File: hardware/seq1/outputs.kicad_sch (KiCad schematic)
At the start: 18 parts, among them J1 AudioJack2_SwitchT, J2 AudioJack2_SwitchT, J4 AudioJack2_SwitchT, U6 TL074

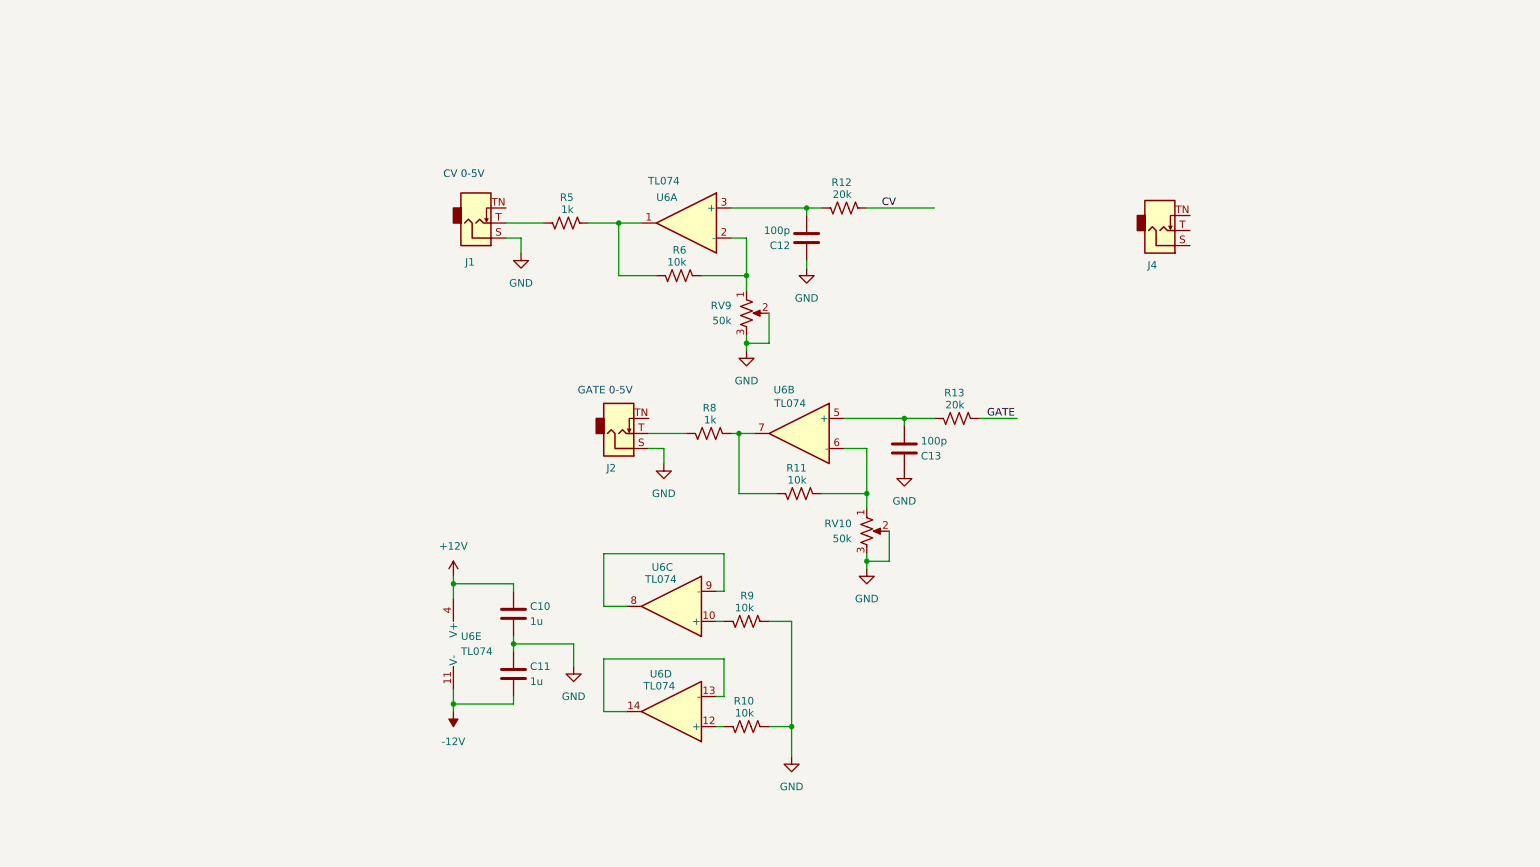
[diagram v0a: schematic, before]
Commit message: schematic and layout for v1 board
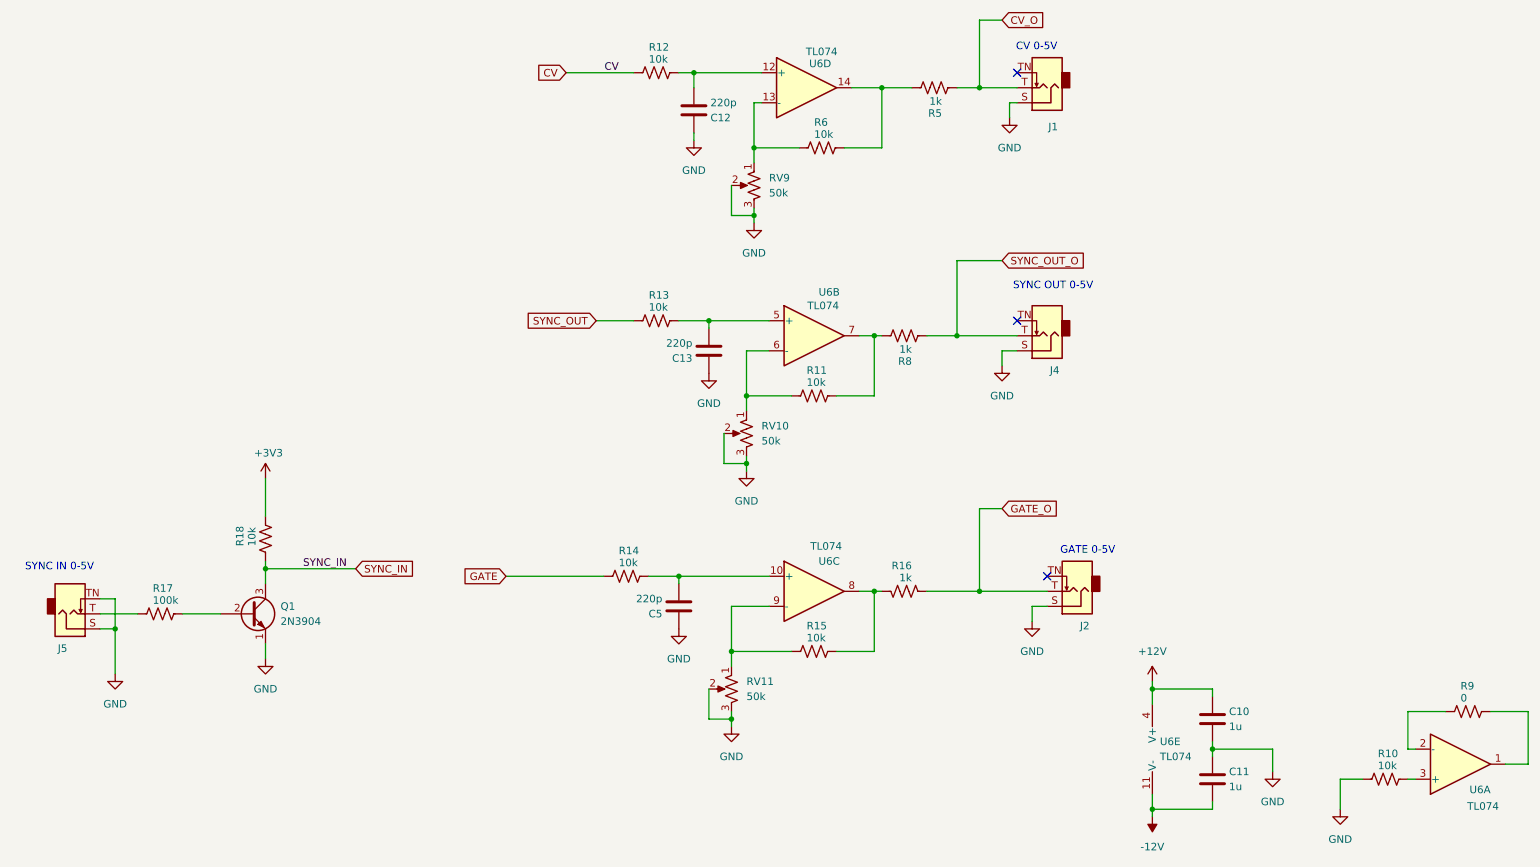
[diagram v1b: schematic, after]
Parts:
- added C5: 220p, Capacitor_THT:C_Disc_D5.0mm_W2.5mm_P5.00mm, symbol Device:C
- added J5: AudioJack2_SwitchT, Connector_Audio_Custom:Mono_Jack_3.5mm_THT_Horizontal, symbol Connector_Audio:AudioJack2_SwitchT
- added Q1: 2N3904, Package_TO_SOT_THT:TO-92_Inline, symbol Transistor_BJT:2N3904
- added R14, R15, R18: 10k, Resistor_THT:R_Axial_DIN0207_L6.3mm_D2.5mm_P2.54mm_Vertical, symbol Device:R_US
- added R16: 1k, Resistor_THT:R_Axial_DIN0207_L6.3mm_D2.5mm_P2.54mm_Vertical, symbol Device:R_US
- added R17: 100k, Resistor_THT:R_Axial_DIN0207_L6.3mm_D2.5mm_P2.54mm_Vertical, symbol Device:R_US
- added RV11: 50k, Potentiometer_THT:Potentiometer_Bourns_3296W_Vertical, symbol Device:R_Potentiometer_US
- C12, C13: value 100p -> 220p
- R12, R13: value 20k -> 10k
- R5: footprint (none) -> Resistor_THT:R_Axial_DIN0207_L6.3mm_D2.5mm_P10.16mm_Horizontal
- R8: footprint (none) -> Resistor_THT:R_Axial_DIN0207_L6.3mm_D2.5mm_P2.54mm_Vertical
- R9: value 10k -> 0
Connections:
- net GATE: now also R14.2; no longer R13.2
- net GND: now also J4.S, C5.1, J5.S, J5.TN, Q1.1 (E), RV11.2, RV11.3; no longer R9.2
- net at R8.1: now also R11.1, U6.7; no longer J2.T
- net at R10.1: now also U6.3 (+); no longer U6.12 (+)
- net at R5.1: now also R6.1, U6.14; no longer J1.T
- net at C12.2, R12.1: now also U6.12 (+); no longer U6.3 (+)
- net at R6.2, RV9.1: now also U6.13 (-); no longer U6.2 (-)
- net at U6.10 (+): now also C5.2, R14.1; no longer R9.1
- net at U6.9 (-): now also R15.2, RV11.1; no longer U6.8
- net SYNC_OUT_O: now reaches J4.T
- net SYNC_OUT_O: now also R8.2
- new net: Q1.2 (B), R17.1
- new net: J5.T, R17.2
- new net: R15.1, R16.1, U6.8
- new net: R9.1, U6.1
- new net: R9.2, U6.2 (-)
- new net +3V3: R18.1
- new net CV_O: J1.T, R5.2
- new net GATE_O: J2.T, R16.2
- new net SYNC_IN: Q1.3 (C), R18.2
- new net SYNC_OUT: R13.2
- no-connect marks 0 -> 3
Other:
- note added: "SYNC IN 0-5V"
- note added: "SYNC OUT 0-5V"
- moved on the sheet: C10, C11, C12, C13, J1, J2, J4, R10, R11, R12, R13, R5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
